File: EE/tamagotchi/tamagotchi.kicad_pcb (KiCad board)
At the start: 4 copper layers, 43.5 x 38.8 mm, 46 parts, among them J1 Conn_01x02_Male, J3 Conn_01x07, J7 TAG_CONNECT, J8 Conn_01x02_Male, P1 USB_C_Plug_USB2.0, Q1 Q_NMOS_GSD, Q2 Q_NMOS_GSD, Q4 Q_NMOS_GSD, SW2 TL1260BQRBLK, SW3 SW_SPDT_321, U1 TPS3840PL30DBVR, U2 STM32G031G8Ux, U3 MPL3115A2, U4 STC4054GR, U5 TPS22919QDCKRQ1, U6 LM3670MF-3.3/NOPB, U8 TPS22919QDCKRQ1

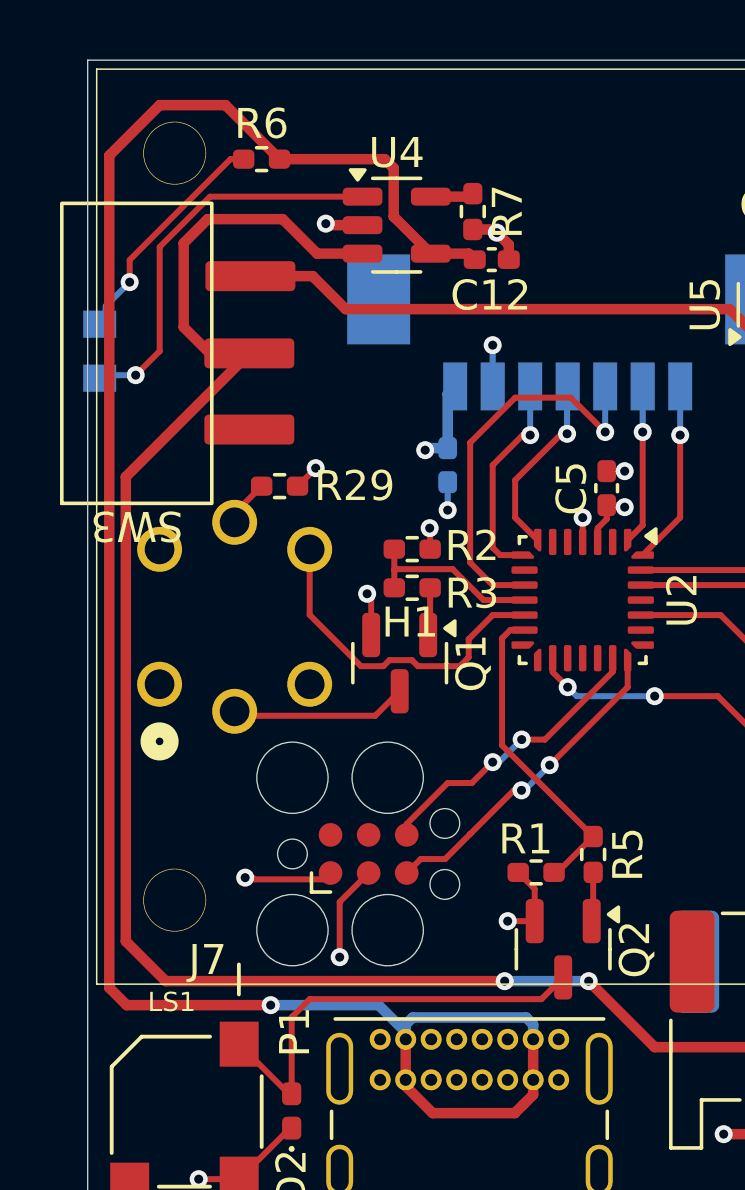
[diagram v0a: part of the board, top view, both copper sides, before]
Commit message: Minor Updates
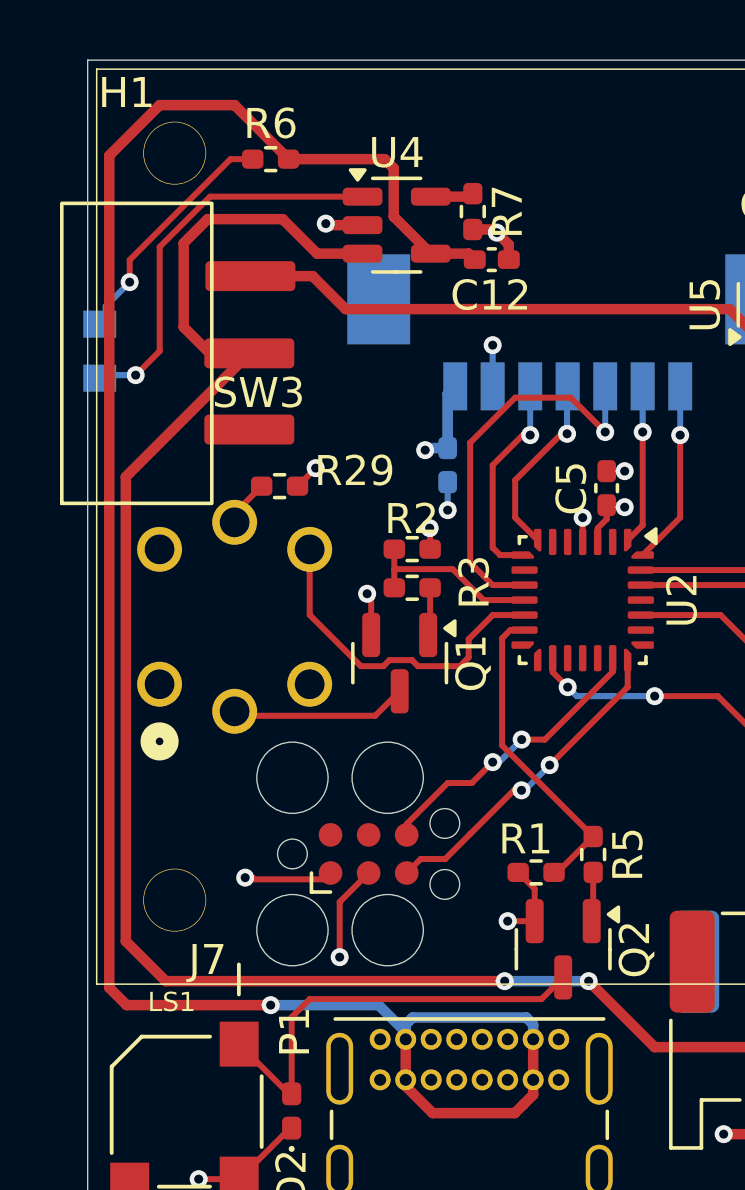
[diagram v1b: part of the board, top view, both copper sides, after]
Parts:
- moved R6 0.30 mm to (142.1, 74.3)
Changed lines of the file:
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@@
 	(footprint "Resistor_SMD:R_0402_1005Metric_Pad0.72x0.64mm_HandSolder"
 		(layer "F.Cu")
-		(at 141.7975 74.3)
+		(at 142.1 74.3)
 		(descr "Resistor SMD 0402 (1005 Metric), square (rectangular) end terminal, IPC-7351 nominal with elongated pad for handsoldering. (Body size source: IPC-SM-782 page 72, https://www.pcb-3d.com/wordpress/wp-content/uploads/ipc-sm-782a_amendment_1_and_2.pdf), generated with kicad-footprint-generator")
 		(tags "resistor handsolder")
@@
 		(tags "resistor handsolder")
 		(property "Reference" "R3"
-			(at 1.9975 0.2 0)
+			(at 2.0825 -0.1875 90)
 			(layer "F.SilkS")
 			(effects
@@
 		(at 136.3 71.3)
 		(property "Reference" "H1"
-			(at 10.45 18.45 0)
+			(at 1 0.8 0)
 			(unlocked yes)
 			(layer "F.SilkS")
@@
 		(tags "resistor handsolder")
 		(property "Reference" "R29"
-			(at -2.5025 0 0)
+			(at -2.5025 0.5 0)
 			(layer "F.SilkS")
 			(effects
@@
 		(tags "resistor handsolder")
 		(property "Reference" "R2"
-			(at 1.9975 -0.1 0)
+			(at -0.017501 -1 0)
 			(layer "F.SilkS")
 			(effects
@@
 		(at 141.387124 80.773785 90)
 		(property "Reference" "SW3"
-			(at -5.75 -3.749999 180)
+			(at -1.326215 0.312876 0)
 			(unlocked yes)
 			(layer "F.SilkS")
@@
 	)
 	(segment
-		(start 142.395 74.3)
-		(end 140.595 72.5)
+		(start 142.1 102.5)
+		(end 137.3 102.5)
 		(width 0.35)
 		(layer "F.Cu")
@@
 	)
 	(segment
-		(start 137.3 102.5)
-		(end 142.1 102.5)
+		(start 136.7199 74.1801)
+		(end 138.4 72.5)
 		(width 0.35)
 		(layer "F.Cu")
@@
 	)
 	(segment
-		(start 145.9 74.3)
-		(end 142.395 74.3)
+		(start 140.8975 72.5)
+		(end 142.6975 74.3)
 		(width 0.35)
 		(layer "F.Cu")
@@
 	)
 	(segment
-		(start 136.7199 101.9199)
-		(end 137.3 102.5)
-		(width 0.35)
-		(layer "F.Cu")
-		(net 10)
-	)
-	(segment
-		(start 138.4 72.5)
-		(end 136.7199 74.1801)
+		(start 148.702498 77.449999)
+		(end 148.9025 77.650001)
 		(width 0.35)
 		(layer "F.Cu")
@@
 	)
 	(segment
-		(start 148.702498 77.449999)
-		(end 148.9025 77.650001)
+		(start 147.4375 77.449999)
+		(end 148.702498 77.449999)
 		(width 0.35)
 		(layer "F.Cu")
@@
 	)
 	(segment
-		(start 147.4375 77.449999)
-		(end 148.702498 77.449999)
+		(start 137.3 102.5)
+		(end 136.7199 101.9199)
 		(width 0.35)
 		(layer "F.Cu")
@@
 	)
 	(segment
-		(start 136.7199 74.1801)
-		(end 136.7199 101.9199)
+		(start 145.9 74.3)
+		(end 142.6975 74.3)
 		(width 0.35)
 		(layer "F.Cu")
@@
 	)
 	(segment
-		(start 140.595 72.5)
-		(end 138.4 72.5)
+		(start 136.7199 101.9199)
+		(end 136.7199 74.1801)
 		(width 0.35)
 		(layer "F.Cu")
@@
 	)
 	(segment
+		(start 138.4 72.5)
+		(end 140.8975 72.5)
+		(width 0.35)
+		(layer "F.Cu")
+		(net 10)
+	)
+	(segment
 		(start 146.201 74.601)
 		(end 145.9 74.3)
@@
 	)
 	(segment
-		(start 140.759734 74.3)
-		(end 137.4 77.659734)
+		(start 137.4 77.659734)
+		(end 140.759734 74.3)
 		(width 0.2)
 		(layer "F.Cu")
@@
 	)
 	(segment
-		(start 137.4 77.659734)
-		(end 137.4 78.4)
+		(start 137.4 78.4)
+		(end 137.4 77.659734)
 		(width 0.2)
 		(layer "F.Cu")
@@
 	)
 	(segment
-		(start 141.2 74.3)
-		(end 140.759734 74.3)
+		(start 140.759734 74.3)
+		(end 141.5025 74.3)
 		(width 0.2)
 		(layer "F.Cu")
